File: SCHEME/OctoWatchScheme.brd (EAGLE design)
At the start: 35 x 34 mm, 23 parts, among them IC1 TP4056, IC2 DS1302, J1 0475900001, Y2 32.768kHz

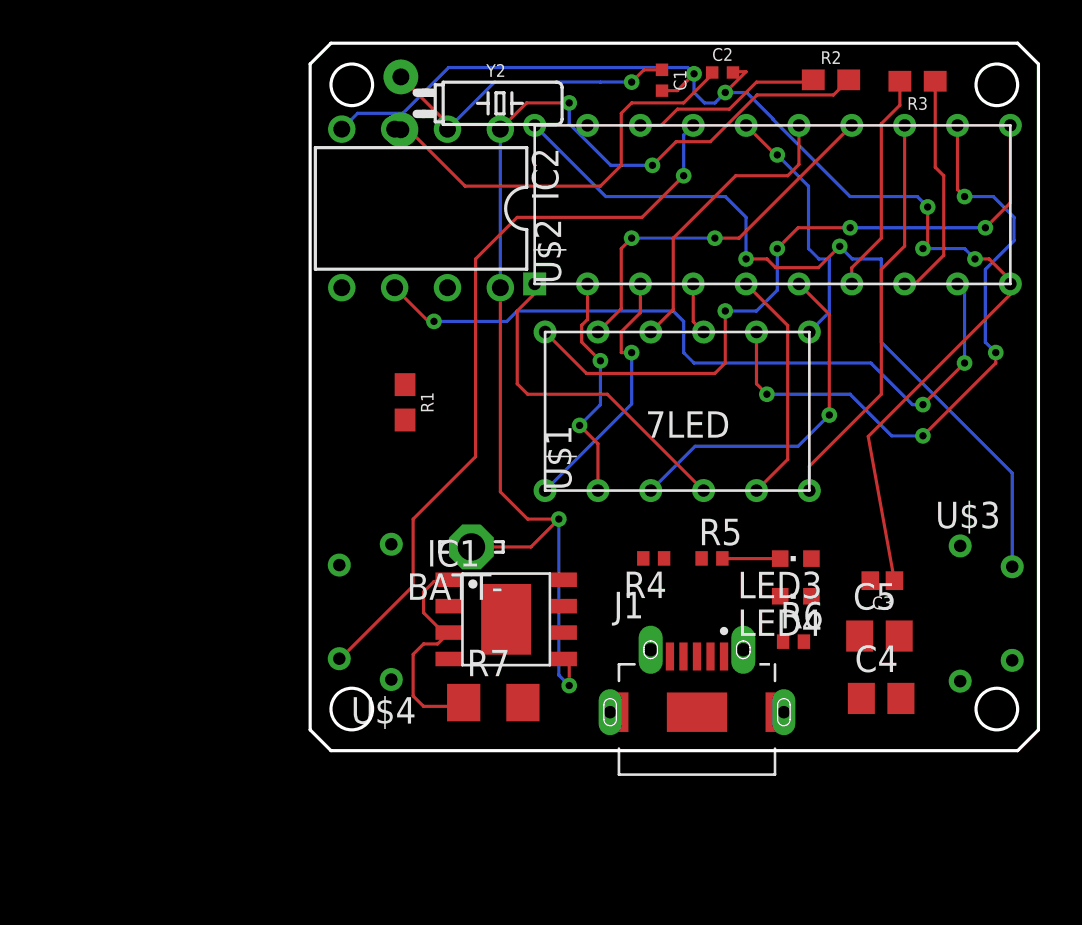
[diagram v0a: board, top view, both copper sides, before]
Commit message: Finalazing scheme
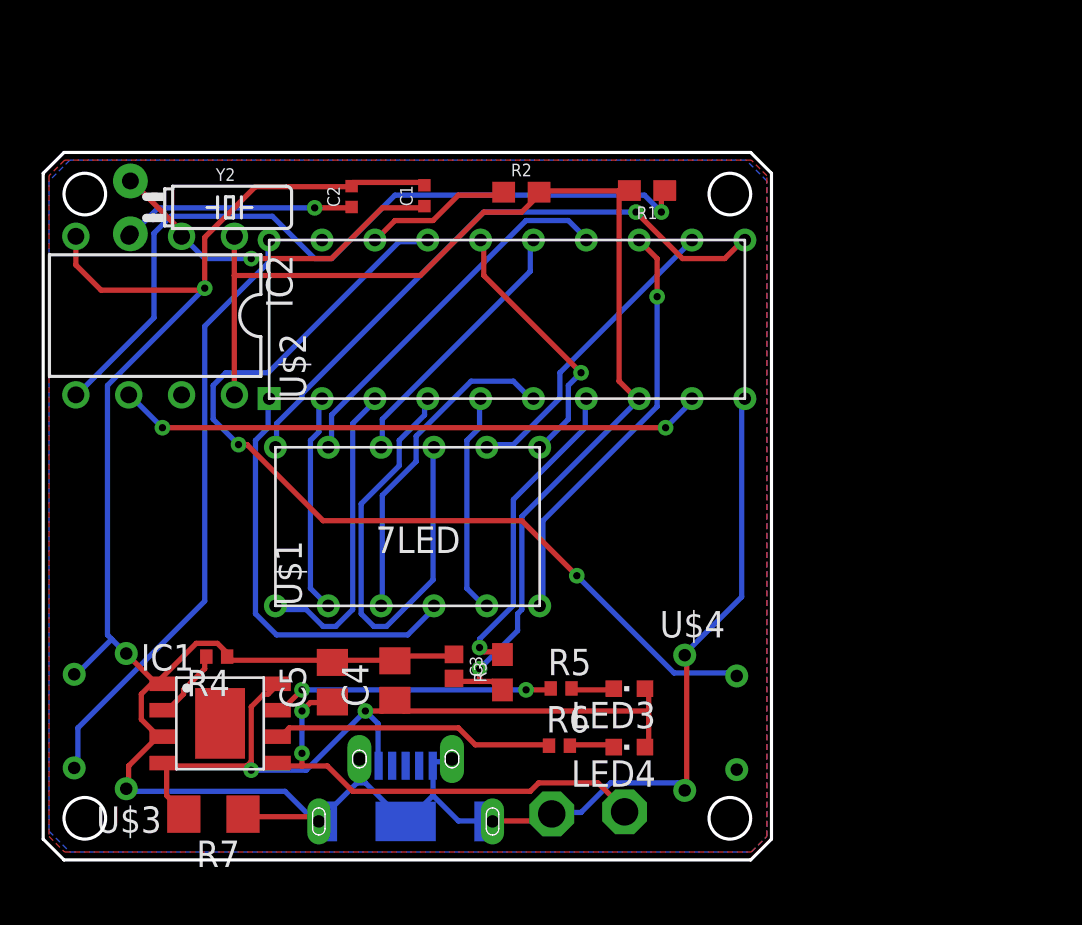
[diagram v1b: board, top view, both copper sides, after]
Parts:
- added BATT+: LSP13, solpad:LSP13
- moved U$3 63.1 mm to (21.7, 32.0), turned to 180 degrees
- moved U$4 38.4 mm to (71.5, 27.5), turned to 0 degrees
- moved R3 34.7 mm to (51.3, 32.1), turned to 90 degrees
- moved C5 26.4 mm to (43.1, 31.7), turned to 90 degrees
- moved C4 23.4 mm to (46.1, 31.7), turned to 90 degrees
- moved R4 21.5 mm to (37.6, 32.9)
- moved C3 21.0 mm to (49.0, 32.4), turned to 270 degrees
- moved C2 18.8 mm to (44.0, 55.0), turned to 90 degrees
- moved R2 15.8 mm to (52.2, 55.2)
- moved R1 15.5 mm to (58.2, 55.3), turned to 180 degrees
- moved J1 15.0 mm to (46.6, 25.0), flipped to the bottom
- moved IC1 14.6 mm to (37.7, 29.7)
- moved R7 14.5 mm to (37.4, 25.3), turned to 180 degrees
- moved U$1 14.1 mm to (48.0, 48.0)
- moved Y2 13.9 mm to (33.4, 54.5)
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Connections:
- removed net N$25: R3.1, U$2.P$8
- removed net VCC: BATT-.MP, C3.2, C5.1, IC1.5, IC2.VCC1, IC2.VCC2, R2.2
- new net BATT+: C3.2, IC2.VCC1, IC2.VCC2, R1.2, R2.2, R3.1, U$2.P$8
- net GND: now also BATT-.MP, U$3.P$3, U$3.P$4, U$4.P$3, U$4.P$4
- net N$18: now also BATT+.MP, C5.1, IC1.5; no longer R1.2
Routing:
- net BATT+: track 0.00 -> 58.7 mm, vias 0 -> 1
- net GND: track 72.6 -> 130.5 mm, vias 5 -> 1
- net VCC: track 55.5 -> 0.00 mm, vias 4 -> 0
- net N$32: track 0.00 -> 38.4 mm, vias 0 -> 2
- net N$17: track 0.00 -> 37.7 mm, vias 0 -> 1
- net N$18: track 0.00 -> 22.3 mm, vias 0 -> 2
- net N$10: track 2.52 -> 22.7 mm
- net N$11: track 30.6 -> 14.7 mm, vias 4 -> 0
- net N$28: track 0.00 -> 13.6 mm, vias 0 -> 2
- net N$26: track 0.00 -> 13.6 mm
- net N$25: track 11.4 -> 0.00 mm
- net N$30: track 38.7 -> 29.3 mm, vias 2 -> 0
- net N$15: track 20.5 -> 11.6 mm, vias 0 -> 1
- net N$19: track 36.5 -> 45.1 mm, vias 1 -> 2
- net N$16: track 35.8 -> 28.4 mm, vias 3 -> 2
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- added copper zone on layer 1, net GND
- added copper zone on layer 16, net GND
